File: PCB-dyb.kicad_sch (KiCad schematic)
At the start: 24 parts, among them J1 Conn_01x10, J2 Conn_01x10, SW1 SW_SPDT, U49 TPS7A20xxxDBV

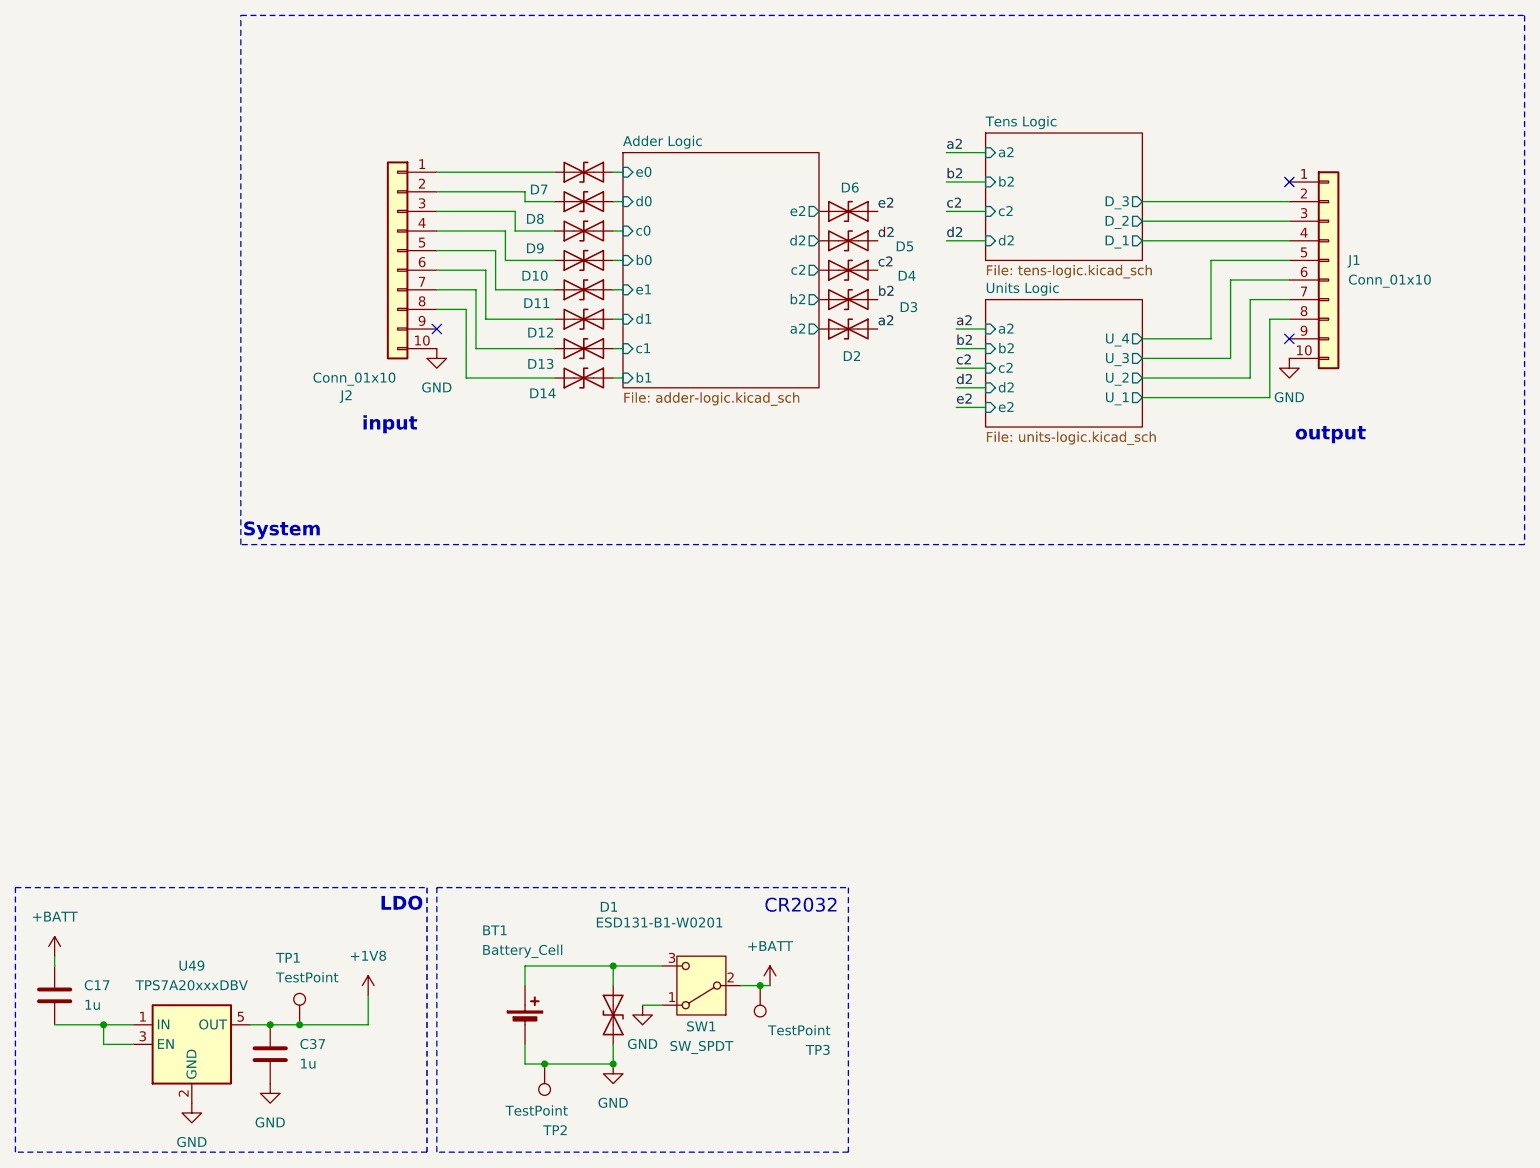
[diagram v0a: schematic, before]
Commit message: ajout composants
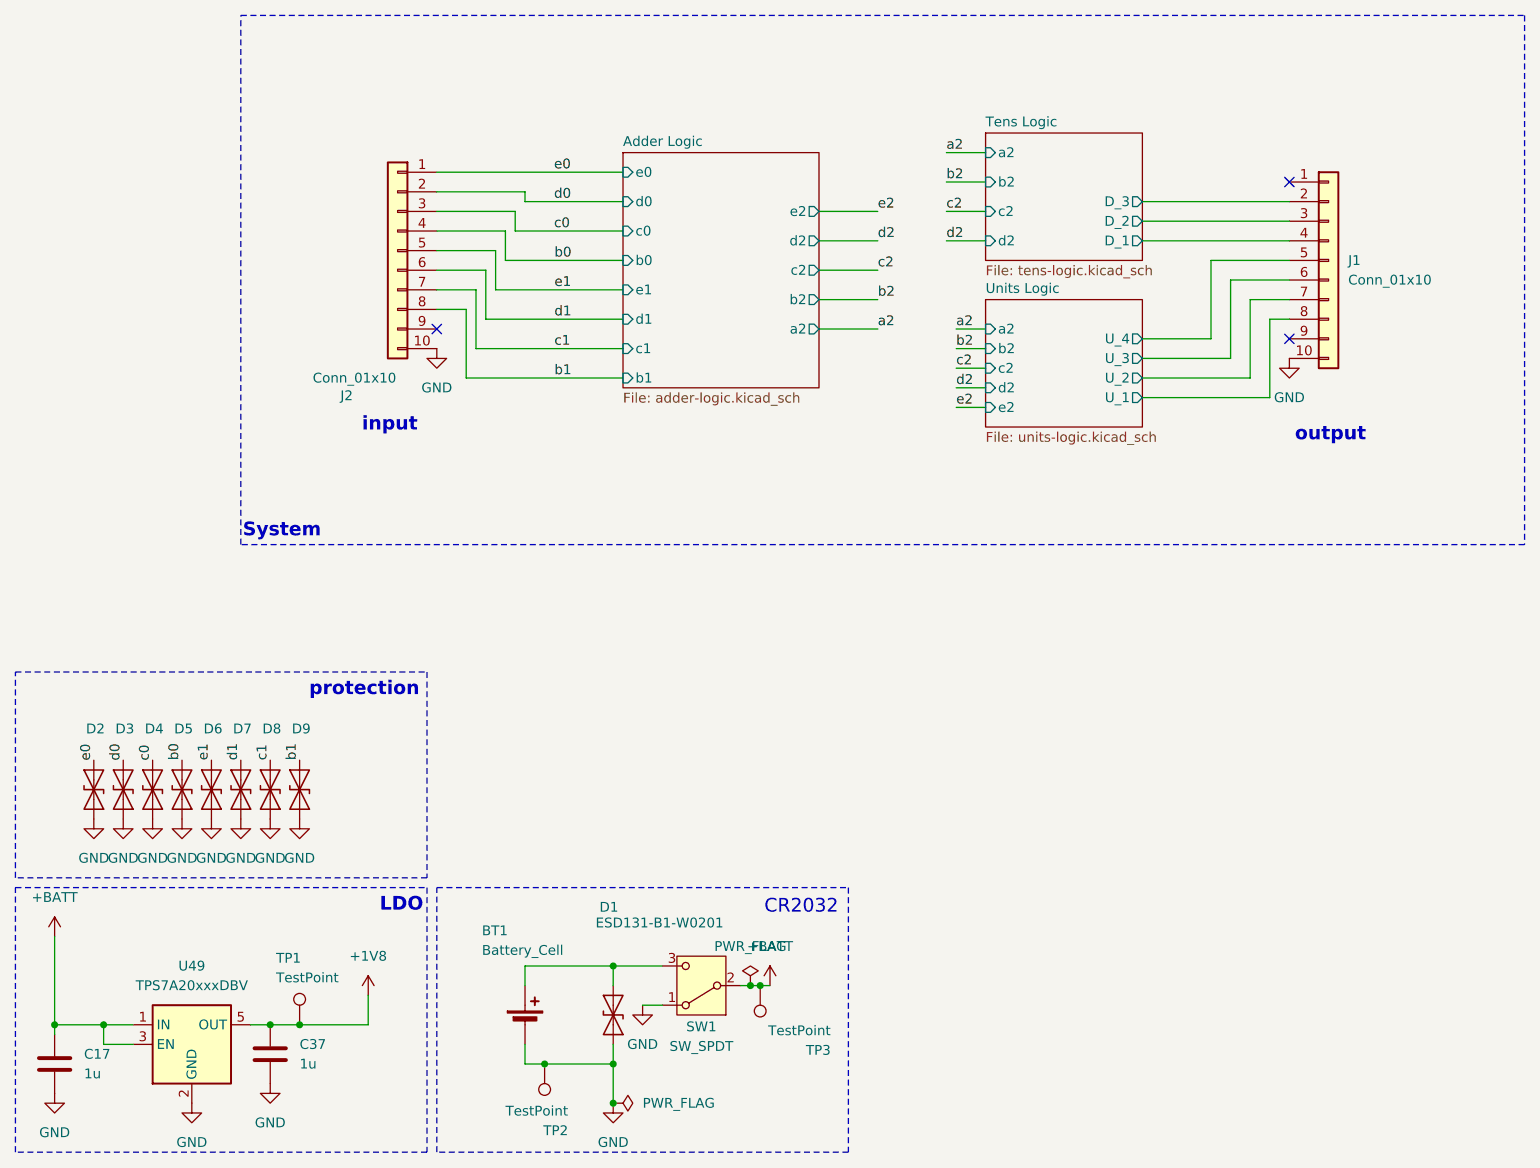
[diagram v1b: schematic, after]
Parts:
- removed D10, D11, D12, D13, D14: ESD131-B1-W0201, Diode_SMD:Infineon_SG-WLL-2-3_0.58x0.28_P0.36mm, symbol Diode:ESD131-B1-W0201
- BT1: Basic (none) -> X; JLCPCB Part # (none) -> C964792; Manufacturer (none) -> MYOUNG; Manufacturer Part Number (none) -> BS-08-B2AA016
- C17, C37: Basic (none) -> Y; JLCPCB Part # (none) -> C1592; Manufacturer (none) -> Samsung Electro-Mechanics; Manufacturer Part Number (none) -> CL10A105KO8NNNC
- D1, D2, D3, D4, D5, D6, D7, D8, D9: Basic (none) -> X; JLCPCB Part # (none) -> C20611048; Manufacturer (none) -> TI; Manufacturer Part Number (none) -> TSD05CDYFR
- SW1: Basic (none) -> X; JLCPCB Part # (none) -> C431540; Manufacturer (none) -> SHOU HAN; Manufacturer Part Number (none) -> MSK12C02
- U49: Basic (none) -> X; JLCPCB Part # (none) -> C963430; Manufacturer (none) -> TI; Manufacturer Part Number (none) -> TPS7A2018PDBVR
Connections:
- net Adder Logic/c0 is gone; now on net GND: D9.1 (A1)
- net Adder Logic/d0 is gone; now on net GND: D8.1 (A1)
- net Adder Logic/d2 is gone; now on net b0: D5.2 (A2)
- net Adder Logic/e0 is gone; now on net GND: D7.1 (A1)
- net Adder Logic/e2 is gone; now on net e1: D6.2 (A2)
- net +BATT: now also U49.1 (IN), U49.3 (EN)
- net GND: now also C17.2, D2.1 (A1), D3.1 (A1), D4.1 (A1), D5.1 (A1), D6.1 (A1)
- net a2: no longer D2.1 (A1)
- net b2: no longer D3.1 (A1)
- net c2: no longer D4.1 (A1)
- net d2: no longer D5.1 (A1)
- net e2: no longer D6.1 (A1)
- net c1: now reaches D8.2 (A2)
- net c1: now also J2.7 (Pin_7); no longer J2.2 (Pin_2)
- net e1: now reaches J2.5 (Pin_5)
- net d1: now reaches D7.2 (A2)
- net d1: now also J2.6 (Pin_6); no longer J2.1 (Pin_1)
- net b1: now reaches D9.2 (A2)
- net b1: now also J2.8 (Pin_8); no longer J2.3 (Pin_3)
- net b0: now reaches J2.4 (Pin_4)
- net Adder Logic/a2: no longer names the net of D2.2 (A2)
- net Adder Logic/b2: no longer names the net of D3.2 (A2)
- net Adder Logic/c2: no longer names the net of D4.2 (A2)
- new net c0: J2.3 (Pin_3)
- new net d0: J2.2 (Pin_2)
- new net e0: J2.1 (Pin_1)
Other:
- note added: "protection"
- moved on the sheet: C17
